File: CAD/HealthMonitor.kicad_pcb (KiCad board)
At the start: 2 copper layers, 70 x 30 mm, 124 parts, among them J1 BAT_T, J10 SDA, J11 SCL, J12 DIS_SW, J13 BAT_CHRG, J14 USBDP, J15 USBDM, J16 USB_V, J17 VBUS, J18 D+, J19 D-, J2 TEG+, J20 SDA, J21 SCL, J22 VCC, J23 GND, J24 BAT_CHRG, J25 DIS_SW, J26 Conn_01x01_Male, J27 MOLEX_51281-0594MOLEX_51281-0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, J28 Conn_01x01_Male, J29 Conn_01x01_Male, J3 TEG-, J4 BAT-, J5 BAT+, J6 USB_C_Receptacle_USB2.0, J7 Conn_02x05_Odd_Even, J8 VCC, J9 GND, U1 MAX17048G+T10, U10 AT24CS02-XHM, U11 BT832L, U12 CP2102N-A01-GQFN24, U13 ADG884BRMZ, U14 LD39015M33R, U2 ADP5092ACPZ-1-R7, U3 LTC4079IDD-PBF, U4 LD39015M33R, U5 BH1792GLC, U6 LSM6DSLTR, U7 TXB0104RUT, U8 MAX1921EUT18+, U9 MAX86141ENP+, Y1 ABS06-32.768KHZ-T

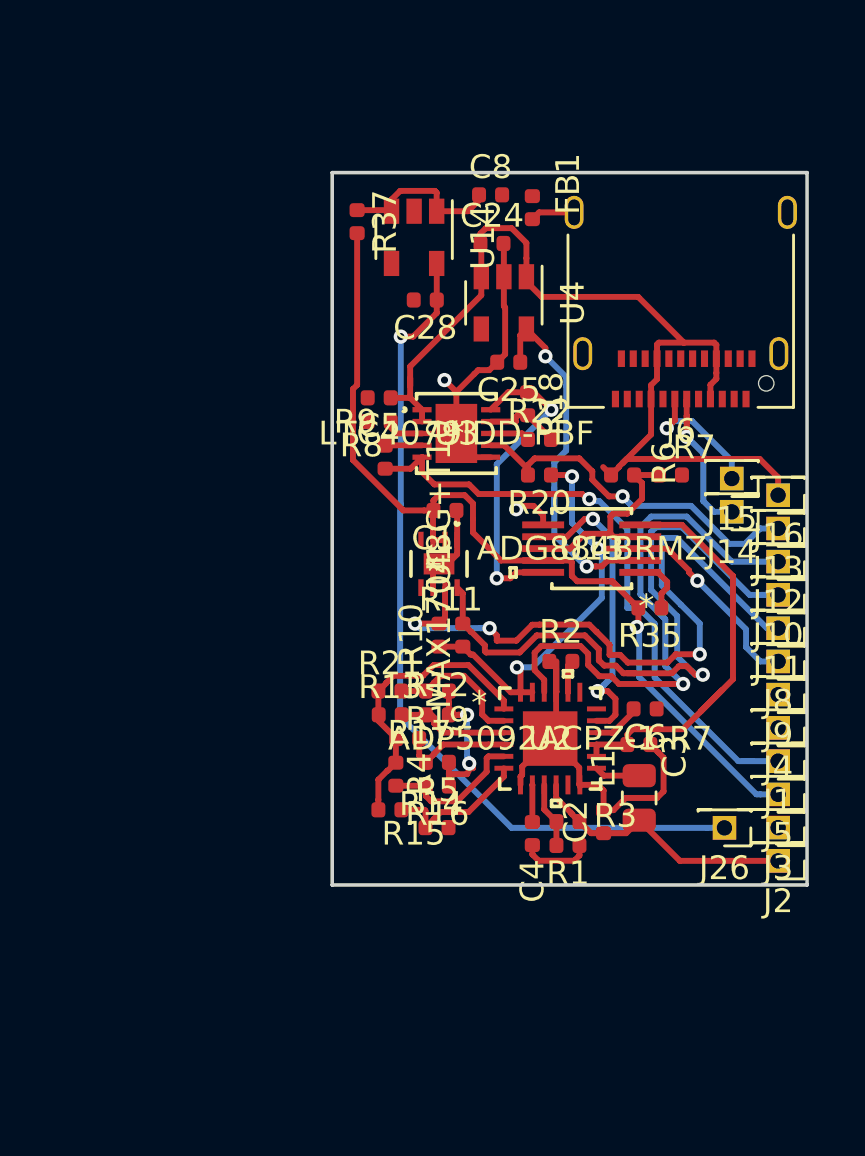
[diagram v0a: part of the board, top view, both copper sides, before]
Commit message: Final version of the firmware code
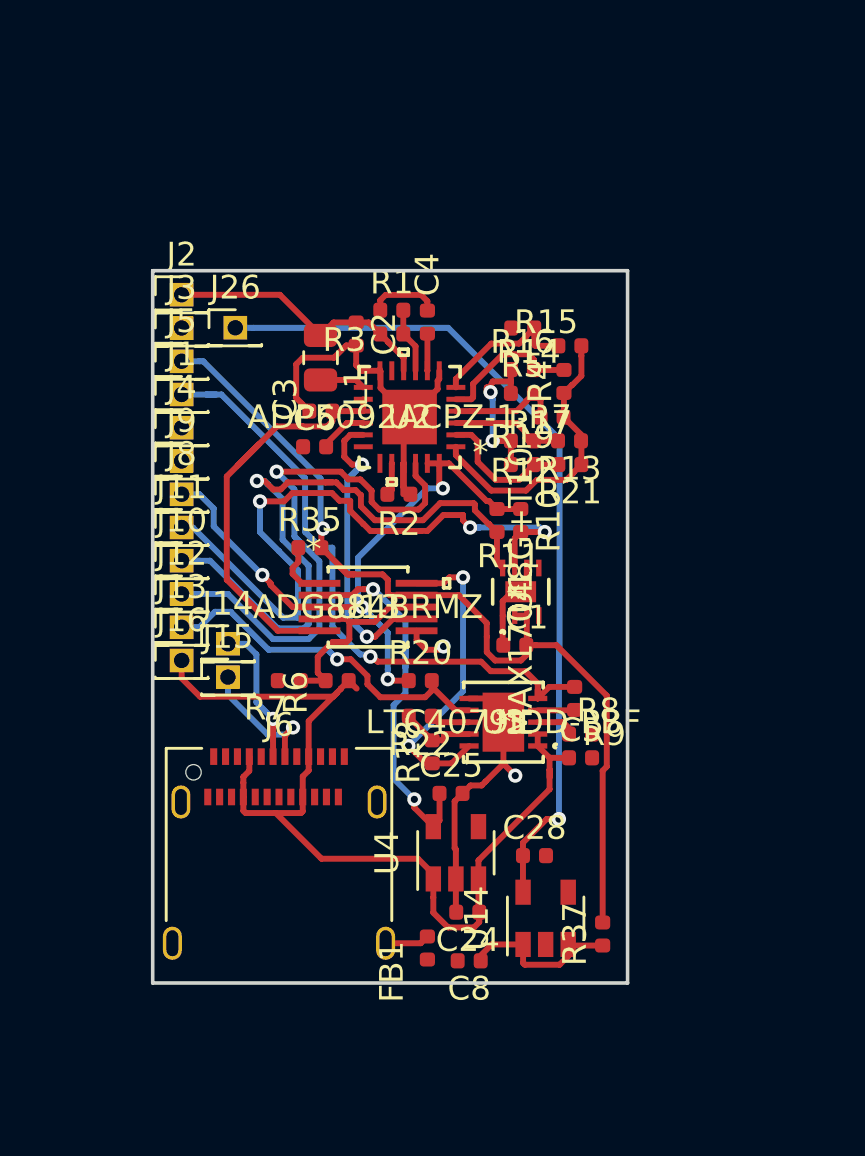
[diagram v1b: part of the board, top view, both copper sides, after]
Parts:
- moved J2 34.6 mm to (143.7, 105.1), turned to 0 degrees
- moved J3 32.8 mm to (143.7, 106.5), turned to 0 degrees
- moved C8 32.3 mm to (155.8, 133.2), turned to 180 degrees
- moved R37 31.7 mm to (161.4, 132.1), turned to 90 degrees
- moved FB1 31.5 mm to (154.0, 132.7), turned to 270 degrees
- moved J5 31.0 mm to (143.7, 107.9), turned to 0 degrees
- moved J6 30.3 mm to (147.8, 129.6), turned to 0 degrees
- moved J1 29.5 mm to (143.7, 109.3), turned to 0 degrees
- moved J26 29.5 mm to (145.9, 106.5), turned to 0 degrees
- moved U14 29.2 mm to (159.0, 131.4), turned to 90 degrees
- moved C24 28.2 mm to (155.7, 131.1), turned to 180 degrees
- moved J4 28.1 mm to (143.7, 110.7), turned to 0 degrees
- moved J9 27.0 mm to (143.7, 112.1), turned to 0 degrees
- moved J8 26.1 mm to (143.7, 113.5), turned to 0 degrees
- moved J16 26.1 mm to (143.7, 120.5), turned to 0 degrees
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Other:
- board size 70 x 30 mm -> 62.4 x 34.1 mm
